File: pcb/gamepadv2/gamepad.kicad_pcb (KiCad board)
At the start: 2 copper layers, 193 x 99.1 mm, 42 parts, among them J1 Arduino Analogs, J2 PiZero2W, J3 SPI0, SW1 Button1, SW2 Button2, SW3 Button3, SW4 Button4, SW5 Rotary1, SW6 Rotary2, SW7 Rotary3, SW8 Rotary4, U1 JOY2, U2 JOY1, U3 MCP3008, U4 MCP3008

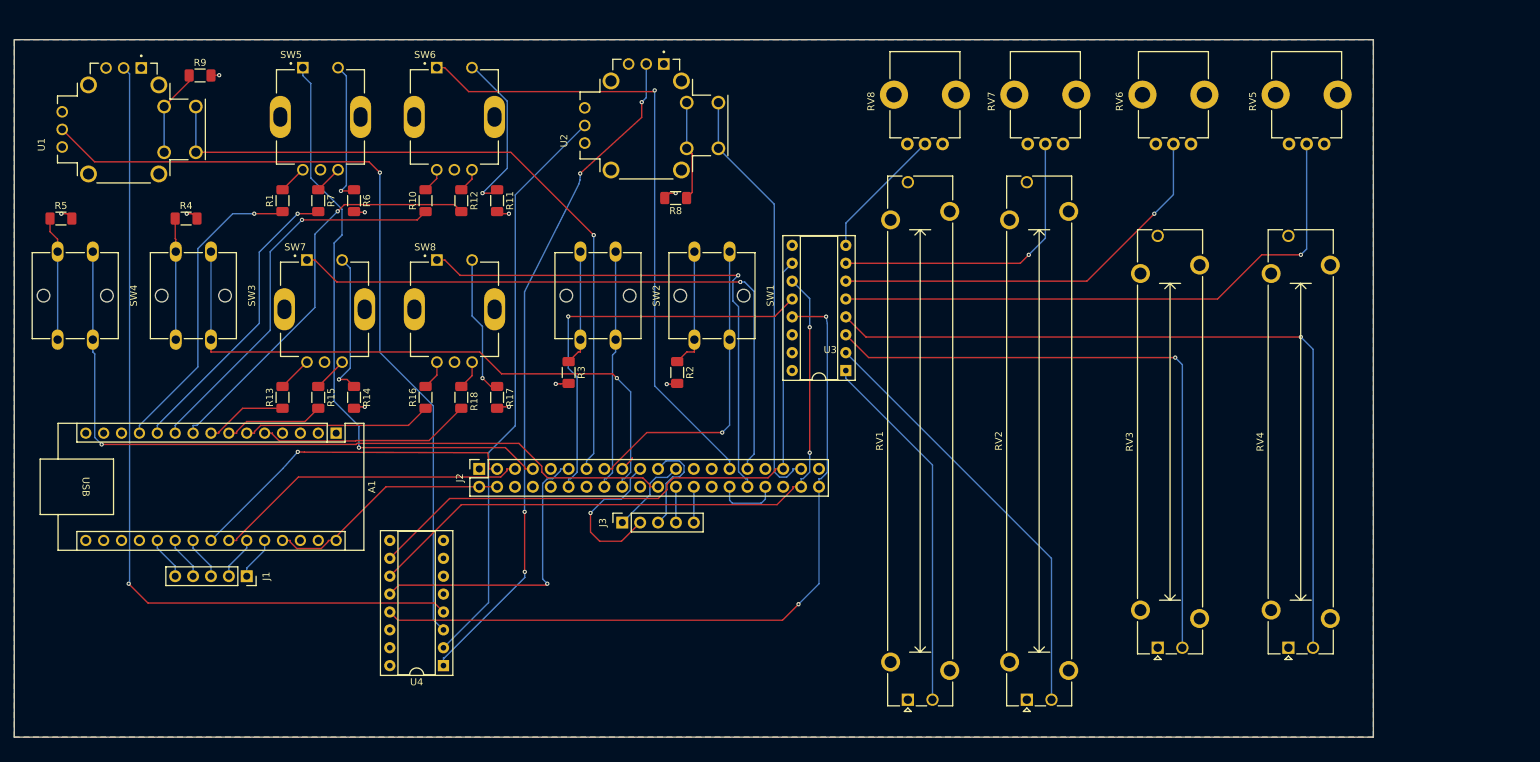
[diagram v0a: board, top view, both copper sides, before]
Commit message: wip
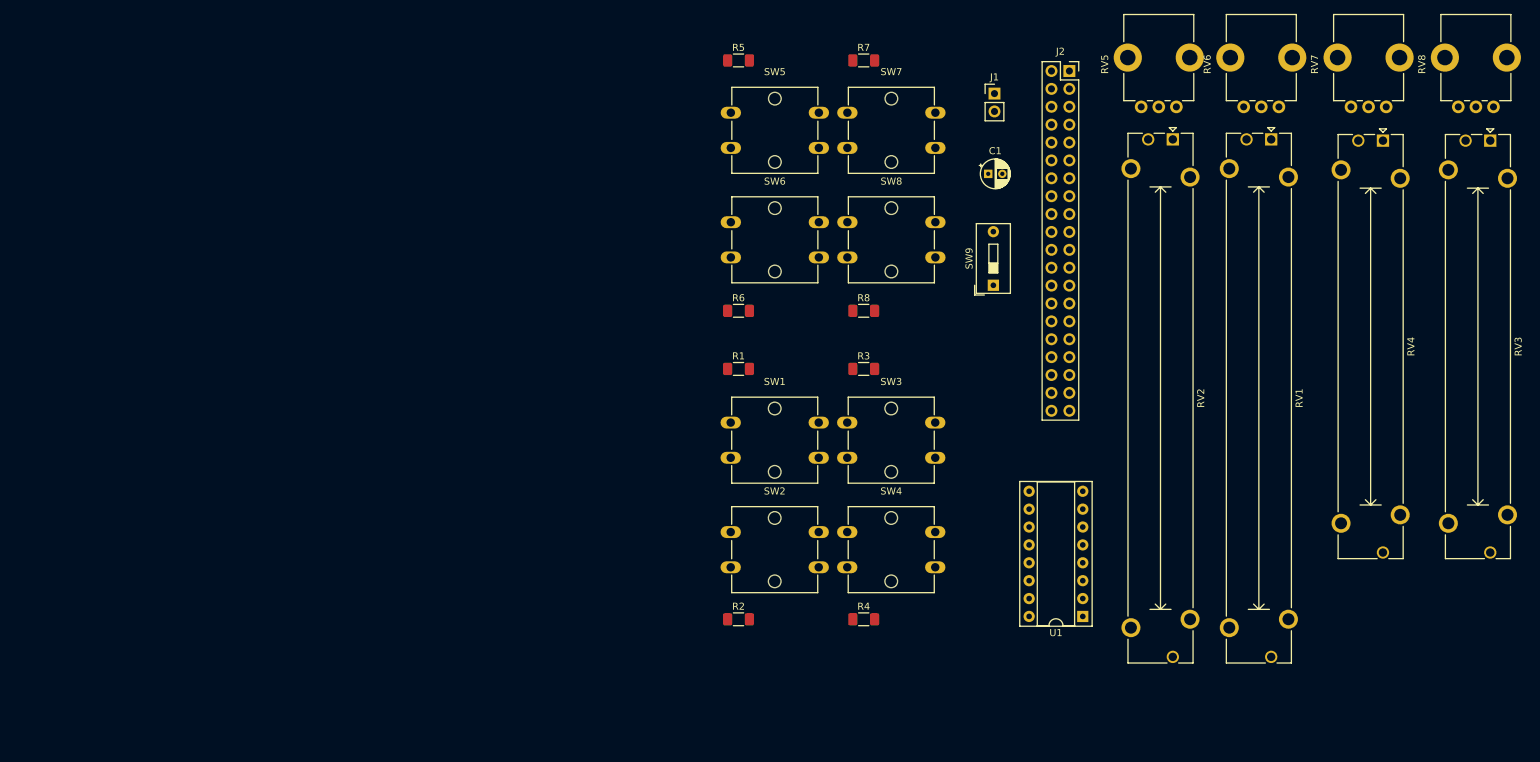
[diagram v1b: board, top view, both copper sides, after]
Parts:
- removed A1: Arduino_Nano_v3.x, Module:Arduino_Nano
- removed J3: SPI0, Connector_PinSocket_2.54mm:PinSocket_1x05_P2.54mm_Vertical
- removed R10, R11, R12, R13, R14, R15, R16, R17, R18, R9: R10K, Resistor_SMD:R_1206_3216Metric_Pad1.30x1.75mm_HandSolder
- removed U2: JOY1, THB001P:CNK_THB001P
- removed U3, U4: MCP3008, Package_DIP:CERDIP-16_W7.62mm_SideBrazed_Socket
- added C1: C_Polarized, Capacitor_THT:CP_Radial_D4.0mm_P2.00mm, F.Cu at (184.1, 67.3)
- added SW9: SW_SPST, Button_Switch_THT:SW_DIP_SPSTx01_Slide_9.78x4.72mm_W7.62mm_P2.54mm, F.Cu at (184.8, 83.1)
- J1: value Arduino Analogs -> PowerConnector; footprint Connector_PinSocket_2.54mm:PinSocket_1x05_P2.54mm_Vertical -> Connector_PinHeader_2.54mm:PinHeader_1x02_P2.54mm_Vertical
- SW5: value Rotary1 -> Button5; footprint PEC11R-4215F-S0024:PEC11R-4215F-S0024 -> Button_Switch_THT:SW_SPST_Omron_B3F-40xx
- SW6: value Rotary2 -> Button6; footprint PEC11R-4215F-S0024:PEC11R-4215F-S0024 -> Button_Switch_THT:SW_SPST_Omron_B3F-40xx
- SW7: value Rotary3 -> Button7; footprint PEC11R-4215F-S0024:PEC11R-4215F-S0024 -> Button_Switch_THT:SW_SPST_Omron_B3F-40xx
- SW8: value Rotary4 -> Button8; footprint PEC11R-4215F-S0024:PEC11R-4215F-S0024 -> Button_Switch_THT:SW_SPST_Omron_B3F-40xx
- U1: value JOY2 -> MCP3008; footprint THB001P:CNK_THB001P -> Package_DIP:CERDIP-16_W7.62mm_SideBrazed_Socket
- moved U1 152.8 mm to (197.5, 130.2), turned to 180 degrees
- moved J1 126.4 mm to (184.9, 55.9), turned to 0 degrees
- moved SW4 114.3 mm to (164.0, 118.2), turned to 0 degrees
- moved R4 111.8 mm to (166.4, 130.6)
- moved J2 101.1 mm to (195.6, 52.7), turned to 0 degrees
- moved R5 98.8 mm to (148.6, 51.2)
- moved RV1 94.8 mm to (224.2, 62.4), turned to -90 degrees
- moved SW3 93.6 mm to (164.0, 102.6), turned to 0 degrees
- moved RV3 86.1 mm to (255.4, 62.6), turned to -90 degrees
- moved RV2 82.2 mm to (210.3, 62.4), turned to -90 degrees
- moved R7 80.0 mm to (166.4, 51.2), turned to 0 degrees
- moved SW7 79.3 mm to (164.1, 58.6)
- moved RV8 78.4 mm to (255.8, 57.8)
- moved RV4 73.3 mm to (240.1, 62.6), turned to -90 degrees
- moved R1 69.0 mm to (148.6, 95.0), turned to 0 degrees
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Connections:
- J1 pad 2: Net-(A1-A6) -> GND
- J2 pad 11: SPI1-CS1 -> unconnected-(J2-GPIO17-Pad11)
- J2 pad 13: JOY-BTN2 -> unconnected-(J2-GPIO27-Pad13)
- J2 pad 19: Net-(J2-MOSI0/GPIO10) -> unconnected-(J2-MOSI0/GPIO10-Pad19)
- J2 pad 21: Net-(J2-MISO0/GPIO9) -> unconnected-(J2-MISO0/GPIO9-Pad21)
- J2 pad 23: Net-(J2-SCLK0/GPIO11) -> unconnected-(J2-SCLK0/GPIO11-Pad23)
- J2 pad 24: Net-(J2-~{CE0}/GPIO8) -> unconnected-(J2-~{CE0}/GPIO8-Pad24)
- J2 pad 26: Net-(J2-~{CE1}/GPIO7) -> unconnected-(J2-~{CE1}/GPIO7-Pad26)
- J2 pad 29: RE-SW3 -> BTN7
- J2 pad 3: Net-(A1-A4) -> unconnected-(J2-SDA/GPIO2-Pad3)
- J2 pad 31: RE-SW2 -> BTN6
- J2 pad 32: RE-SW1 -> BTN5
- J2 pad 36: SPI1-CS2 -> unconnected-(J2-GPIO16-Pad36)
- J2 pad 37: JOY-BTN1 -> unconnected-(J2-GPIO26-Pad37)
- J2 pad 5: Net-(A1-A5) -> unconnected-(J2-SCL/GPIO3-Pad5)
- J2 pad 7: RE-SW4 -> BTN8
- R1 pad 1: Net-(A1-D9) -> Net-(R1-Pad1)
- R1 pad 2: Net-(R1-Pad2) -> GND
- R7 pad 2: Net-(A1-D8) -> GND
- RV1 pad 2: Net-(U3-CH0) -> Net-(U1-CH0)
- RV2 pad 2: Net-(U3-CH1) -> Net-(U1-CH1)
- RV3 pad 2: Net-(U3-CH2) -> Net-(U1-CH2)
- RV4 pad 2: Net-(U3-CH3) -> Net-(U1-CH3)
- RV5 pad 2: Net-(U3-CH4) -> Net-(U1-CH4)
- RV6 pad 2: Net-(U3-CH5) -> Net-(U1-CH5)
- RV7 pad 2: Net-(U3-CH6) -> Net-(U1-CH6)
- RV8 pad 2: Net-(U3-CH7) -> Net-(U1-CH7)
- SW1 pad 2: Net-(R2-Pad1) -> Net-(R1-Pad1)
- SW2 pad 2: Net-(R3-Pad1) -> Net-(R2-Pad1)
- SW3 pad 2: Net-(R4-Pad1) -> Net-(R3-Pad1)
- SW4 pad 2: Net-(R5-Pad1) -> Net-(R4-Pad1)
- SW5 pad 1: RE-SW4 -> BTN5
- SW5 pad 2: Net-(R6-Pad1) -> Net-(R5-Pad1)
- SW6 pad 1: RE-SW3 -> BTN6
- SW6 pad 2: Net-(R11-Pad1) -> Net-(R6-Pad1)
- SW7 pad 1: RE-SW2 -> BTN7
- SW7 pad 2: Net-(R14-Pad1) -> Net-(R7-Pad1)
- SW8 pad 1: RE-SW1 -> BTN8
- SW8 pad 2: Net-(R17-Pad1) -> Net-(R8-Pad1)
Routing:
- net Net-(U4-CH3): track 120.0 -> 0.00 mm, vias 1 -> 0
- net Net-(U4-CH2): track 116.3 -> 0.00 mm, vias 1 -> 0
- net Net-(U3-CH3): track 110.7 -> 0.00 mm, vias 1 -> 0
- net BTN4: track 110.2 -> 0.00 mm, vias 1 -> 0
- net SPI1-CLK: track 107.1 -> 0.00 mm, vias 2 -> 0
- net JOY-BTN2: track 101.5 -> 0.00 mm, vias 1 -> 0
- net Net-(U4-CH0): track 96.3 -> 0.00 mm, vias 4 -> 0
- net SPI1-MOSI: track 95.0 -> 0.00 mm, vias 2 -> 0
- net SPI1-MISO: track 91.5 -> 0.00 mm
- net RE-SW2: track 91.0 -> 0.00 mm, vias 1 -> 0
- net RE-SW3: track 90.6 -> 0.00 mm, vias 1 -> 0
- net BTN3: track 90.3 -> 0.00 mm, vias 1 -> 0
- net Net-(U3-CH2): track 89.8 -> 0.00 mm, vias 1 -> 0
- net RE-SW4: track 84.3 -> 0.00 mm, vias 1 -> 0
- net Net-(U3-CH4): track 83.3 -> 0.00 mm, vias 1 -> 0
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- removed copper zone on F.Cu, net 3V3
- removed copper zone on B.Cu, net GND
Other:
- board outline removed

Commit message: wip
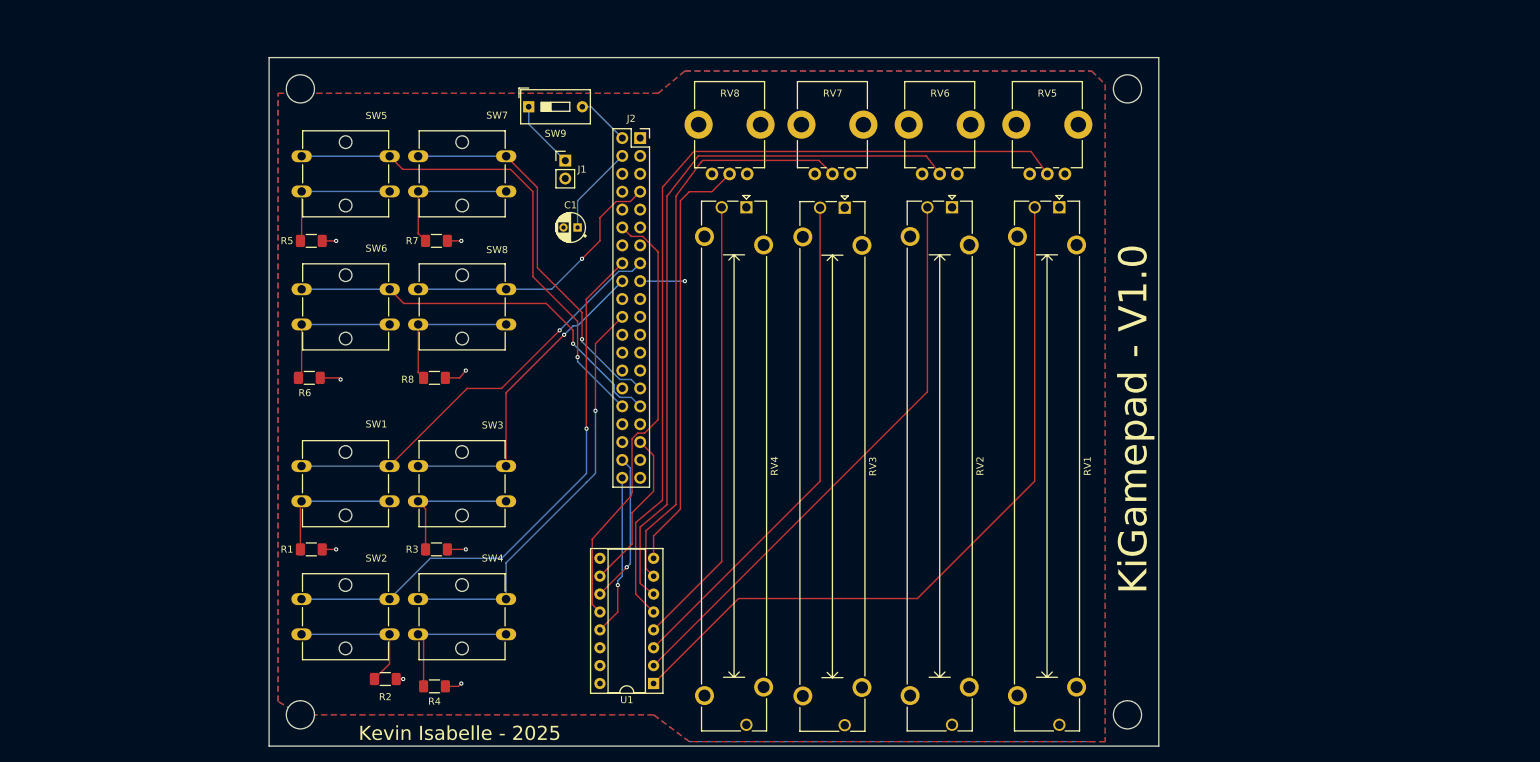
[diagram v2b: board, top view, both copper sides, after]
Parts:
- added REF**: MountingHole_4mm, MountingHole:MountingHole_4mm, F.Cu at (203.8, 144.1)
- added REF**: MountingHole_4mm, MountingHole:MountingHole_4mm, F.Cu at (86.4, 144.1)
- added REF**: MountingHole_4mm, MountingHole:MountingHole_4mm, F.Cu at (203.8, 55.2)
- added REF**: MountingHole_4mm, MountingHole:MountingHole_4mm, F.Cu at (86.4, 55.2)
- RV3, RV4: footprint Potentiometer_THT:Potentiometer_Bourns_PTA4543_Single_Slide -> Potentiometer_THT:Potentiometer_Bourns_PTA6043_Single_Slide
- moved RV8 106.4 mm to (149.8, 67.3)
- moved RV3 92.2 mm to (163.7, 72.1)
- moved RV4 90.9 mm to (149.7, 72.1)
- moved RV7 76.7 mm to (164.4, 67.3)
- moved SW9 70.7 mm to (118.8, 57.8), turned to 0 degrees
- moved R1 65.9 mm to (87.9, 120.7)
- moved R3 65.9 mm to (105.7, 120.7)
- moved R5 65.9 mm to (87.9, 76.8)
- moved R7 65.9 mm to (105.7, 76.8)
- moved J2 61.7 mm to (134.6, 62.2)
- moved R4 61.7 mm to (105.4, 140.1)
- moved R6 61.7 mm to (87.6, 96.3)
- moved R8 61.7 mm to (105.4, 96.3)
- moved SW4 61.7 mm to (103.1, 127.7)
- moved SW8 61.7 mm to (103.1, 83.7)
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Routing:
- net Net-(U1-CH4): track 0.00 -> 121.7 mm
- net Net-(U1-CH0): track 0.00 -> 104.9 mm
- net Net-(U1-CH5): track 0.00 -> 102.0 mm
- net Net-(U1-CH6): track 0.00 -> 82.0 mm
- net Net-(U1-CH1): track 0.00 -> 81.2 mm
- net BTN2: track 0.00 -> 79.9 mm, vias 0 -> 1
- net Net-(U1-CH2): track 0.00 -> 72.3 mm
- net BTN5: track 0.00 -> 70.7 mm, vias 0 -> 1
- net Net-(U1-CH3): track 0.00 -> 64.0 mm
- net SPI1-CS0: track 0.00 -> 62.4 mm
- net Net-(U1-CH7): track 0.00 -> 60.9 mm
- net BTN1: track 0.00 -> 60.0 mm, vias 0 -> 1
- net BTN4: track 0.00 -> 59.4 mm, vias 0 -> 1
- net BTN6: track 0.00 -> 56.7 mm, vias 0 -> 1
- net BTN7: track 0.00 -> 54.3 mm, vias 0 -> 1
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- added copper zone on F.Cu, net 3V3
- added copper zone on B.Cu, net GND
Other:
- board outline added: 126.4 x 97.8 mm
- board text added: "Kevin Isabelle - 2025"
- board text added: "KiGamepad - V1.0"
